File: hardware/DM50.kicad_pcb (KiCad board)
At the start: 2 copper layers, 70 x 149.5 mm, 99 parts, among them J1 ST-LINK, J2 USB_C_Receptacle_USB2.0_14P, Q1 MMBT3904, SW10 CST, SW11 VAR, SW12 U, SW13 NXT, SW14 quote, SW15 STO, SW16 EVAL, SW17 L, SW18 D, SW19 R, SW2 F1, SW20 SIN, SW21 COS, SW22 TAN, SW23 SQR, SW24 y^x, SW25 1/x, SW26 ENTER, SW27 ENTER, SW28 +/-, SW29 EEX, SW3 F2, SW30 DEL, SW31 BACK, SW32 ALPHA, SW33 7, SW34 8, SW35 9, SW36 /, SW37 OPT1, SW38 4, SW39 5, SW4 F3, SW40 6, SW41 x, SW42 RESET, SW43 OPT2, SW44 1, SW45 2, SW46 3, SW47 -, SW48 ON, SW49 0, SW5 F4, SW50 ., SW51 SPC, SW52 +, SW6 F5, SW7 F6, SW8 MTH, SW9 PRG, U1 EA_DOGL128X-6, U2 STM32U535CBT6, U3 AT25SF641, U4 USBLC6-2SC6, U5 ADP2108AUJ-3.3, Y1 HSE 16MHz

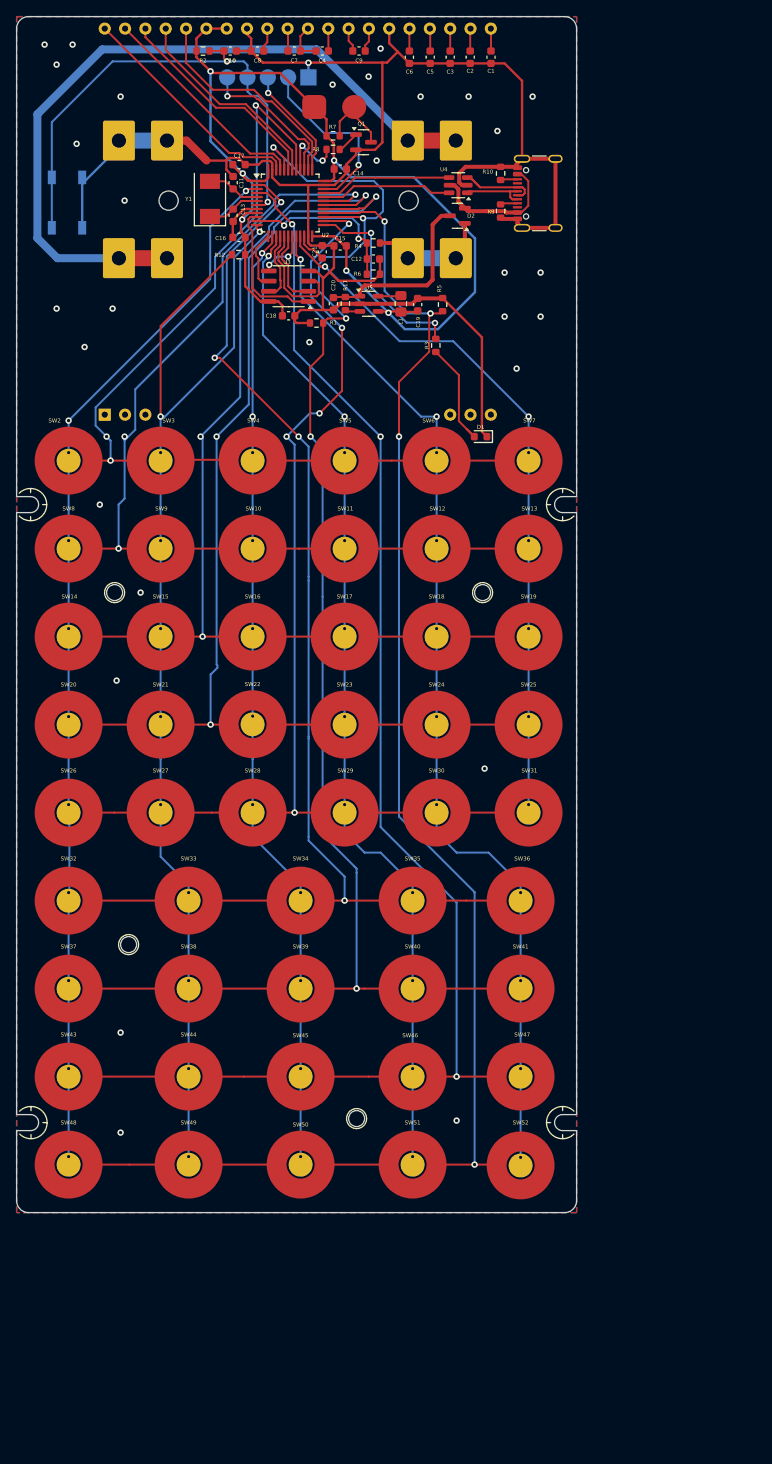
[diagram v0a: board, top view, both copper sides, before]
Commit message: pcb changes
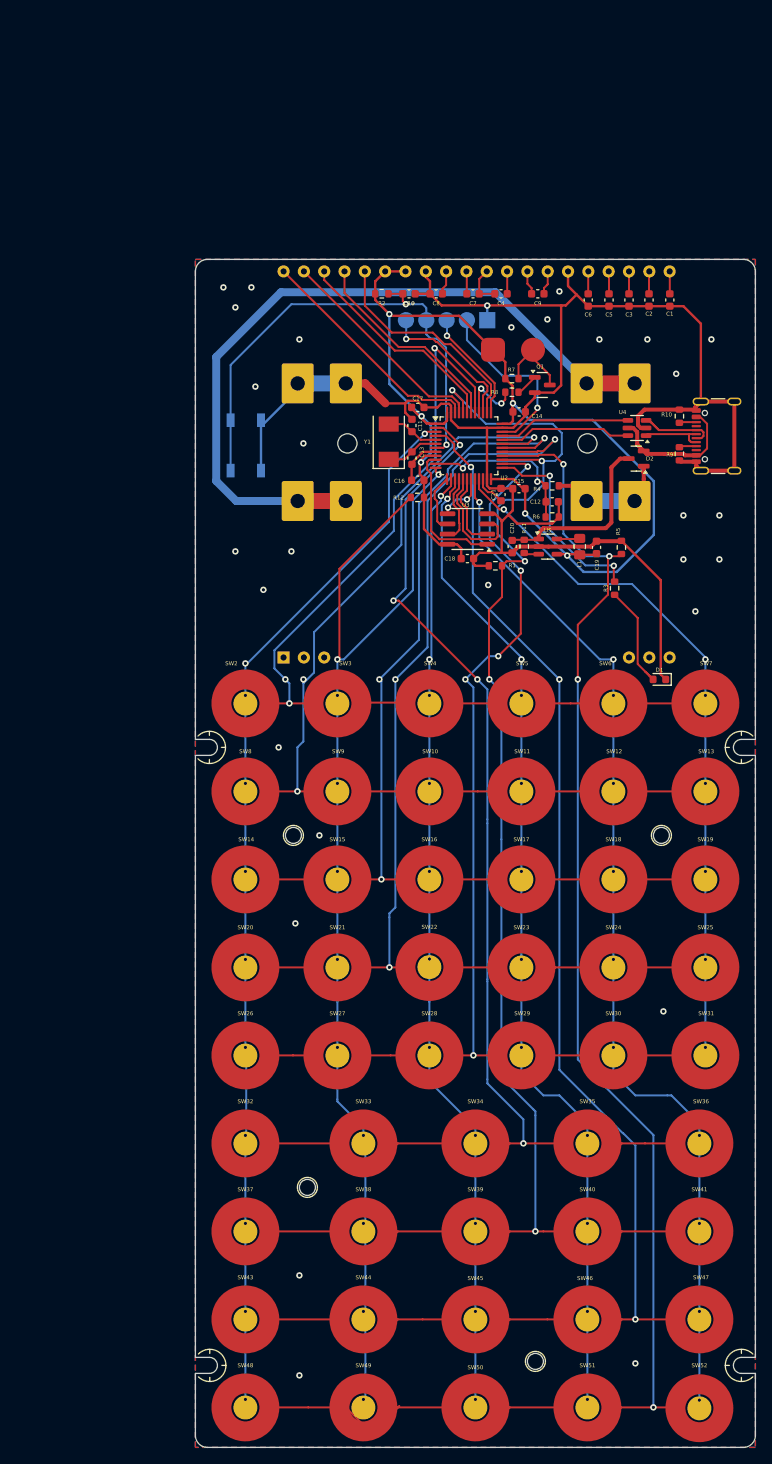
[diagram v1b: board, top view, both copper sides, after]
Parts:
- moved C12 37.7 mm to (116.0, 93.2)
- moved C8 37.7 mm to (101.5, 67.2)
- moved C9 37.7 mm to (114.2, 67.2)
- moved R2 37.7 mm to (94.7, 67.2)
- moved R4 37.7 mm to (116.0, 91.2)
- moved BZ1 37.7 mm to (111.0, 74.2)
- moved C10 37.7 mm to (98.0, 67.2)
- moved C16 37.7 mm to (99.2, 90.5)
- moved C4 37.7 mm to (109.5, 67.2)
- moved C7 37.7 mm to (106.0, 67.2)
- moved D2 37.7 mm to (126.5, 87.8)
- moved R1 37.7 mm to (108.8, 101.2)
- moved R3 37.7 mm to (123.8, 104.0)
- moved R9 37.7 mm to (131.8, 87.2)
- moved U2 37.7 mm to (105.5, 86.2)
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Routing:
- net COL02: track 149.7 -> 150.2 mm
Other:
- board size 70 x 149.5 mm -> 70 x 148.5 mm
